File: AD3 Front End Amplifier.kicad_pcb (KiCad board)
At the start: 4 copper layers, 72.4 x 65.4 mm, 50 parts, among them IC101 XC6901D501MR-G, J101 CH1, J102 CH2, J103 W1, J104 W2, J105 Conn_01x15_Pin, J106 Conn_01x15_Socket, J107 Conn_01x15_Pin, J108 Conn_01x15_Socket, SW101 AC/DC, SW102 AC/DC, SW103 50, SW104 50, U101 MIC5504-2.5YM5, U102 OPA356xxDBV, U103 OPA356xxDBV, U104 OPA356xxDBV, U105 OPA356xxDBV

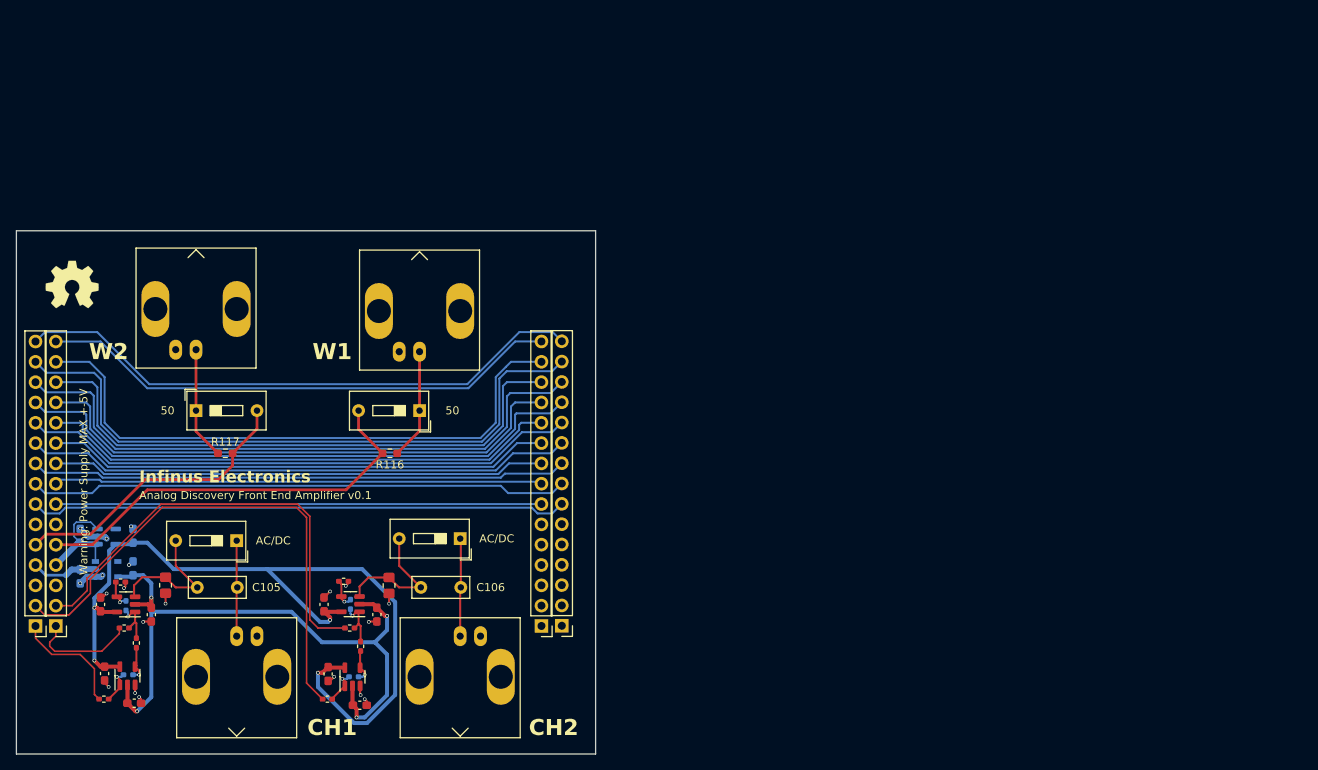
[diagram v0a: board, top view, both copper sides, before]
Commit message: v2 gerbers and pdf schematics
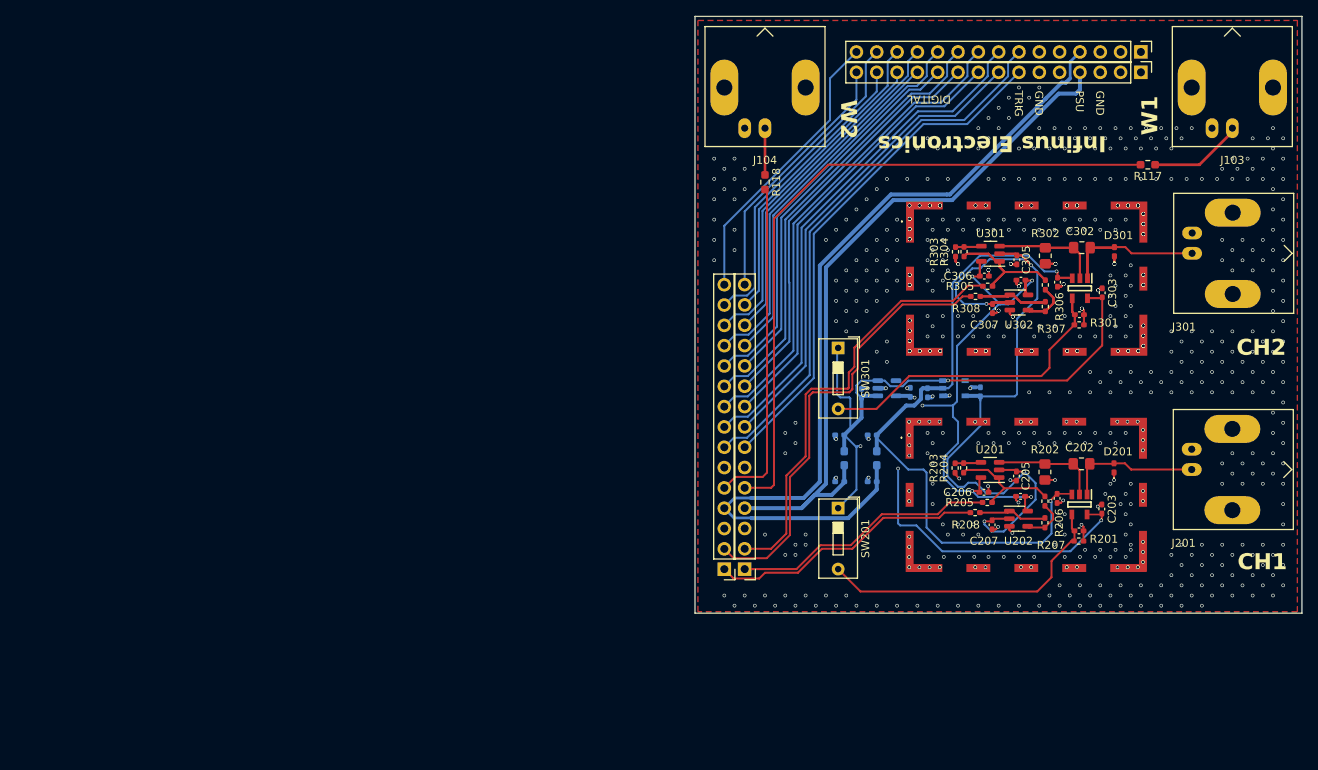
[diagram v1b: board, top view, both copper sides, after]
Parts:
- removed C101, C102, C109, C110, C111, C112, C113, C114, C115, C116: 10u, Capacitor_SMD:C_0603_1608Metric_Pad1.08x0.95mm_HandSolder
- removed C105, C106: 10n, Capacitor_THT:C_Rect_L7.0mm_W2.5mm_P5.00mm
- removed C107, C108: 1u, Capacitor_SMD:C_0603_1608Metric_Pad1.08x0.95mm_HandSolder
- removed IC101: XC6901D501MR-G, XC6901:SOT95P280X130-5N
- removed J101: CH1, Connector_Coaxial:BNC_Amphenol_B6252HB-NPP3G-50_Horizontal
- removed J102: CH2, Connector_Coaxial:BNC_Amphenol_B6252HB-NPP3G-50_Horizontal
- removed R102, R103: 1M, Resistor_SMD:R_0805_2012Metric_Pad1.20x1.40mm_HandSolder
- removed R104, R105: 100, Resistor_SMD:R_0402_1005Metric_Pad0.72x0.64mm_HandSolder
- removed R106, R107, R109, R111, R112, R113: 402, Resistor_SMD:R_0402_1005Metric_Pad0.72x0.64mm_HandSolder
- removed R108, R110, R114, R115: 22, Resistor_SMD:R_0402_1005Metric_Pad0.72x0.64mm_HandSolder
- removed R116: 49.9, Resistor_SMD:R_0603_1608Metric_Pad0.98x0.95mm_HandSolder
- removed the REF** at (96.3, 95.8)
- removed the REF** at (99.6, 146.8)
- removed SW101, SW102: AC/DC, Button_Switch_THT:SW_DIP_SPSTx01_Slide_9.78x4.72mm_W7.62mm_P2.54mm
- removed SW103, SW104: 50, Button_Switch_THT:SW_DIP_SPSTx01_Slide_9.78x4.72mm_W7.62mm_P2.54mm
- removed U101: MIC5504-2.5YM5, Package_TO_SOT_SMD:SOT-23-5
- removed U102, U103, U104: OPA356xxDBV, Package_TO_SOT_SMD:SOT-23-5
- added C117: 1u, Capacitor_SMD:C_0402_1005Metric_Pad0.74x0.62mm_HandSolder, B.Cu at (203.2, 109.3)
- added C118: 1u, Capacitor_SMD:C_0402_1005Metric_Pad0.74x0.62mm_HandSolder, B.Cu at (194.9, 109.3)
- added C119: 1u, Capacitor_SMD:C_0402_1005Metric_Pad0.74x0.62mm_HandSolder, B.Cu at (201.0, 109.2)
- added C120: 1u, Capacitor_SMD:C_0402_1005Metric_Pad0.74x0.62mm_HandSolder, B.Cu at (209.8, 109.2)
- added C121: 1u, Capacitor_SMD:C_0402_1005Metric_Pad0.74x0.62mm_HandSolder, B.Cu at (196.3, 120.4)
- added C122: 1u, Capacitor_SMD:C_0402_1005Metric_Pad0.74x0.62mm_HandSolder, B.Cu at (196.3, 114.6)
- added C123: 1u, Capacitor_SMD:C_0402_1005Metric_Pad0.74x0.62mm_HandSolder, B.Cu at (192.2, 120.4)
- added C124: 1u, Capacitor_SMD:C_0402_1005Metric_Pad0.74x0.62mm_HandSolder, B.Cu at (192.2, 114.6)
- added C201: 10n, Capacitor_SMD:C_0402_1005Metric_Pad0.74x0.62mm_HandSolder, F.Cu at (222.1, 126.5)
- added C202: 10n, Capacitor_SMD:C_0805_2012Metric_Pad1.18x1.45mm_HandSolder, F.Cu at (222.4, 118.2)
- added C203: 1u, Capacitor_SMD:C_0402_1005Metric_Pad0.74x0.62mm_HandSolder, F.Cu at (225.0, 123.8)
- added C204: 1u, Capacitor_SMD:C_0402_1005Metric_Pad0.74x0.62mm_HandSolder, F.Cu at (219.4, 122.5)
- added C205: 1u, Capacitor_SMD:C_0402_1005Metric_Pad0.74x0.62mm_HandSolder, F.Cu at (214.3, 119.7)
- added C206: 1u, Capacitor_SMD:C_0402_1005Metric_Pad0.74x0.62mm_HandSolder, F.Cu at (210.3, 121.7)
- added C207: 1u, Capacitor_SMD:C_0402_1005Metric_Pad0.74x0.62mm_HandSolder, F.Cu at (211.3, 125.8)
- added C208: 1u, Capacitor_SMD:C_0402_1005Metric_Pad0.74x0.62mm_HandSolder, F.Cu at (214.8, 122.2)
- added C301: 10n, Capacitor_SMD:C_0402_1005Metric_Pad0.74x0.62mm_HandSolder, F.Cu at (222.2, 99.5)
- added C302: 10n, Capacitor_SMD:C_0805_2012Metric_Pad1.18x1.45mm_HandSolder, F.Cu at (222.5, 91.1)
- added C303: 1u, Capacitor_SMD:C_0402_1005Metric_Pad0.74x0.62mm_HandSolder, F.Cu at (225.0, 96.8)
- added C304: 1u, Capacitor_SMD:C_0402_1005Metric_Pad0.74x0.62mm_HandSolder, F.Cu at (219.4, 95.5)
- added C305: 1u, Capacitor_SMD:C_0402_1005Metric_Pad0.74x0.62mm_HandSolder, F.Cu at (214.4, 92.7)
- added C306: 1u, Capacitor_SMD:C_0402_1005Metric_Pad0.74x0.62mm_HandSolder, F.Cu at (210.3, 94.7)
- added C307: 1u, Capacitor_SMD:C_0402_1005Metric_Pad0.74x0.62mm_HandSolder, F.Cu at (211.3, 98.8)
- added C308: 1u, Capacitor_SMD:C_0402_1005Metric_Pad0.74x0.62mm_HandSolder, F.Cu at (214.9, 95.2)
- added D201: D_TVS, Diode_SMD:D_0402_1005Metric_Pad0.77x0.64mm_HandSolder, F.Cu at (226.5, 118.7)
- added D301: D_TVS, Diode_SMD:D_0402_1005Metric_Pad0.77x0.64mm_HandSolder, F.Cu at (226.6, 91.6)
- added FB101: FerriteBead_Small, Inductor_SMD:L_0603_1608Metric_Pad1.05x0.95mm_HandSolder, B.Cu at (196.8, 117.5)
- added FB102: FerriteBead_Small, Inductor_SMD:L_0603_1608Metric_Pad1.05x0.95mm_HandSolder, B.Cu at (192.8, 117.5)
- added H201: SMS-409F, SMS409:SMS409F, F.Cu at (215.5, 122.0)
- added H301: SMS-409F, SMS409:SMS409F, F.Cu at (215.6, 95.0)
- added IC103: XC6901D501MR-G, XC6901:SOT95P280X130-5N, B.Cu at (206.5, 108.7)
- added IC201: TS12A4516DBVR, TS12A4516:SOT95P280X145-5N, F.Cu at (222.2, 123.2)
- added IC301: TS12A4516DBVR, TS12A4516:SOT95P280X145-5N, F.Cu at (222.2, 96.2)
- added J201: CH1, Connector_Coaxial:BNC_Amphenol_B6252HB-NPP3G-50_Horizontal, F.Cu at (236.2, 118.9)
- added J301: CH1, Connector_Coaxial:BNC_Amphenol_B6252HB-NPP3G-50_Horizontal, F.Cu at (236.3, 91.8)
- added R118: 49.9, Resistor_SMD:R_0603_1608Metric_Pad0.98x0.95mm_HandSolder, F.Cu at (182.9, 83.0)
- added R201: 1k, Resistor_SMD:R_0402_1005Metric_Pad0.72x0.64mm_HandSolder, F.Cu at (222.1, 127.8)
- added R202: 1M, Resistor_SMD:R_0805_2012Metric_Pad1.20x1.40mm_HandSolder, F.Cu at (217.9, 119.2)
- added R203: 100, Resistor_SMD:R_0402_1005Metric_Pad0.72x0.64mm_HandSolder, F.Cu at (206.6, 118.7)
- added R204: 402, Resistor_SMD:R_0402_1005Metric_Pad0.72x0.64mm_HandSolder, F.Cu at (207.7, 118.7)
- added R205: 22, Resistor_SMD:R_0402_1005Metric_Pad0.72x0.64mm_HandSolder, F.Cu at (210.7, 123.0)
- added R206: 402, Resistor_SMD:R_0402_1005Metric_Pad0.72x0.64mm_HandSolder, F.Cu at (217.9, 122.8)
- added R207: 402, Resistor_SMD:R_0402_1005Metric_Pad0.72x0.64mm_HandSolder, F.Cu at (217.9, 125.5)
- added R208: 22, Resistor_SMD:R_0402_1005Metric_Pad0.72x0.64mm_HandSolder, F.Cu at (209.1, 124.3)
- added R301: 1k, Resistor_SMD:R_0402_1005Metric_Pad0.72x0.64mm_HandSolder, F.Cu at (222.2, 100.8)
- added R302: 1M, Resistor_SMD:R_0805_2012Metric_Pad1.20x1.40mm_HandSolder, F.Cu at (217.9, 92.2)
- added R303: 100, Resistor_SMD:R_0402_1005Metric_Pad0.72x0.64mm_HandSolder, F.Cu at (206.7, 91.7)
- added R304: 402, Resistor_SMD:R_0402_1005Metric_Pad0.72x0.64mm_HandSolder, F.Cu at (207.8, 91.6)
- added R305: 22, Resistor_SMD:R_0402_1005Metric_Pad0.72x0.64mm_HandSolder, F.Cu at (210.7, 96.0)
- added R306: 402, Resistor_SMD:R_0402_1005Metric_Pad0.72x0.64mm_HandSolder, F.Cu at (217.9, 95.8)
- added R307: 402, Resistor_SMD:R_0402_1005Metric_Pad0.72x0.64mm_HandSolder, F.Cu at (217.9, 98.5)
- added R308: 22, Resistor_SMD:R_0402_1005Metric_Pad0.72x0.64mm_HandSolder, F.Cu at (209.2, 97.2)
- added REF**: OSHW-Logo2_7.3x6mm_SilkScreen, Symbol:OSHW-Logo2_7.3x6mm_SilkScreen, B.Cu at (197.2, 76.1)
- added REF**: KiCad-Logo2_5mm_SilkScreen, Symbol:KiCad-Logo2_5mm_SilkScreen, B.Cu at (224.2, 76.3)
- added SW201: AC/DC, Button_Switch_THT:SW_DIP_SPSTx01_Slide_9.78x4.72mm_W7.62mm_P2.54mm, F.Cu at (192.0, 123.7)
- added SW301: AC/DC, Button_Switch_THT:SW_DIP_SPSTx01_Slide_9.78x4.72mm_W7.62mm_P2.54mm, F.Cu at (192.0, 103.7)
- added U201: OPA356xxDBV, Package_TO_SOT_SMD:SOT-23-5, F.Cu at (211.0, 118.9)
- added U202: OPA356xxDBV, Package_TO_SOT_SMD:SOT-23-5, F.Cu at (214.6, 125.0)
- added U301: OPA356xxDBV, Package_TO_SOT_SMD:SOT-23-5, F.Cu at (211.1, 91.9)
- added U302: OPA356xxDBV, Package_TO_SOT_SMD:SOT-23-5, F.Cu at (214.6, 98.0)
- U105: value OPA356xxDBV -> MIC5504-2.5YM5; moved to B.Cu
- moved R117 120.8 mm to (230.7, 80.8), turned to 180 degrees
- moved J103 105.4 mm to (241.3, 76.2)
- moved J107 102.0 mm to (229.9, 69.2), turned to -90 degrees
- moved J105 101.9 mm to (229.9, 66.7), turned to -90 degrees
- moved J108 86.4 mm to (180.3, 131.3)
- moved J106 86.4 mm to (177.8, 131.3)
- moved J104 76.3 mm to (182.9, 76.2)
- moved U105 75.9 mm to (198.1, 108.7), turned to 0 degrees
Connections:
- net /V+ renamed /V+_CONN
- net /V- renamed /V-_CONN
- J106 pad 1: /CH1_OUT- -> CH1_OUT-
- J106 pad 2: /CH2_OUT- -> CH2_OUT-
- J108 pad 1: /CH1_OUT+ -> CH1_OUT+
- J108 pad 2: /CH2_OUT+ -> CH2_OUT+
- R117 pad 1: Net-(J104-In) -> Net-(J103-In)
- R117 pad 2: /W2 -> /W1
- U105 pad 1: Net-(R113-Pad1) -> V+
- U105 pad 2: -2V5 -> GND
- U105 pad 3: GND -> V+
- U105 pad 4: Net-(U105--) -> unconnected-(U105-NC-Pad4)
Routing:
- net V+: track 0.00 -> 123.8 mm, vias 0 -> 4
- net V-: track 0.00 -> 86.2 mm, vias 0 -> 2
- net /CH2_OUT-: track 65.0 -> 0.00 mm
- net /CH2_OUT+: track 56.3 -> 0.00 mm
- net CH2_OUT-: track 0.00 -> 56.2 mm
- net CH2_OUT+: track 0.00 -> 54.7 mm
- net Net-(IC301-IN): track 0.00 -> 42.2 mm
- net /D14: track 80.7 -> 40.5 mm
- net /D6: track 75.3 -> 35.9 mm
- net Net-(IC201-IN): track 0.00 -> 37.9 mm
- net /D15: track 72.1 -> 35.9 mm
- net +2V5: track 104.9 -> 69.6 mm, vias 4 -> 6
- net CH1_OUT-: track 0.00 -> 34.6 mm
- net /W1: track 52.2 -> 85.7 mm
- net /D5: track 73.0 -> 39.5 mm
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- added copper zone on F.Cu, net GND
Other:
- board size 72.4 x 65.4 mm -> 75.9 x 74.6 mm
- board text added: "AD3 Low Noise Amplifier v0.2"
- board text added: "CH1"
- board text added: "CH2"
- board text added: "DIGITAL"
- board text added: "GND"
- board text added: "PSU"
- board text added: "TRIG"
- board text added: "W1"
- board text added: "W2"
- board text removed: "Analog Discovery Front End Amplifier v0.1"
- board text removed: "Warning: Power Supply MAX +-5V"
